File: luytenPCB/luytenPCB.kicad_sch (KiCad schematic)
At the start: 36 parts, among them IC1 DRV8212DRLR, IC2 DRV8212DRLR, J1 Battery, J10 START_M, J2 BDC1, J3 BDC2, J4 LINE_RF, J5 LINE_LF, J6 DIST_L, J7 DIST_LM, J8 DIST_R, J9 DIST_RM, SW1 SW_SPST, SW2 ProgSelect

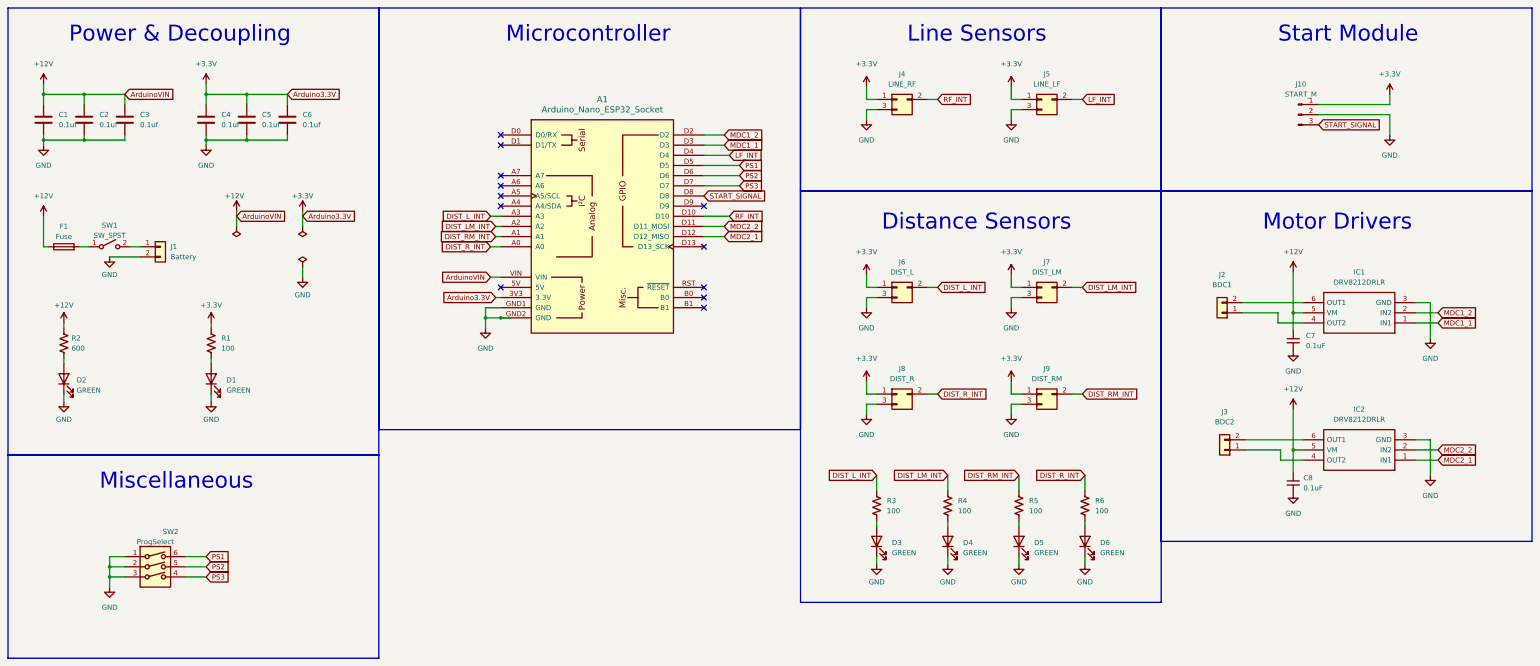
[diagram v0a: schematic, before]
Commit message: pcb production prototype done
finished schematic and layout
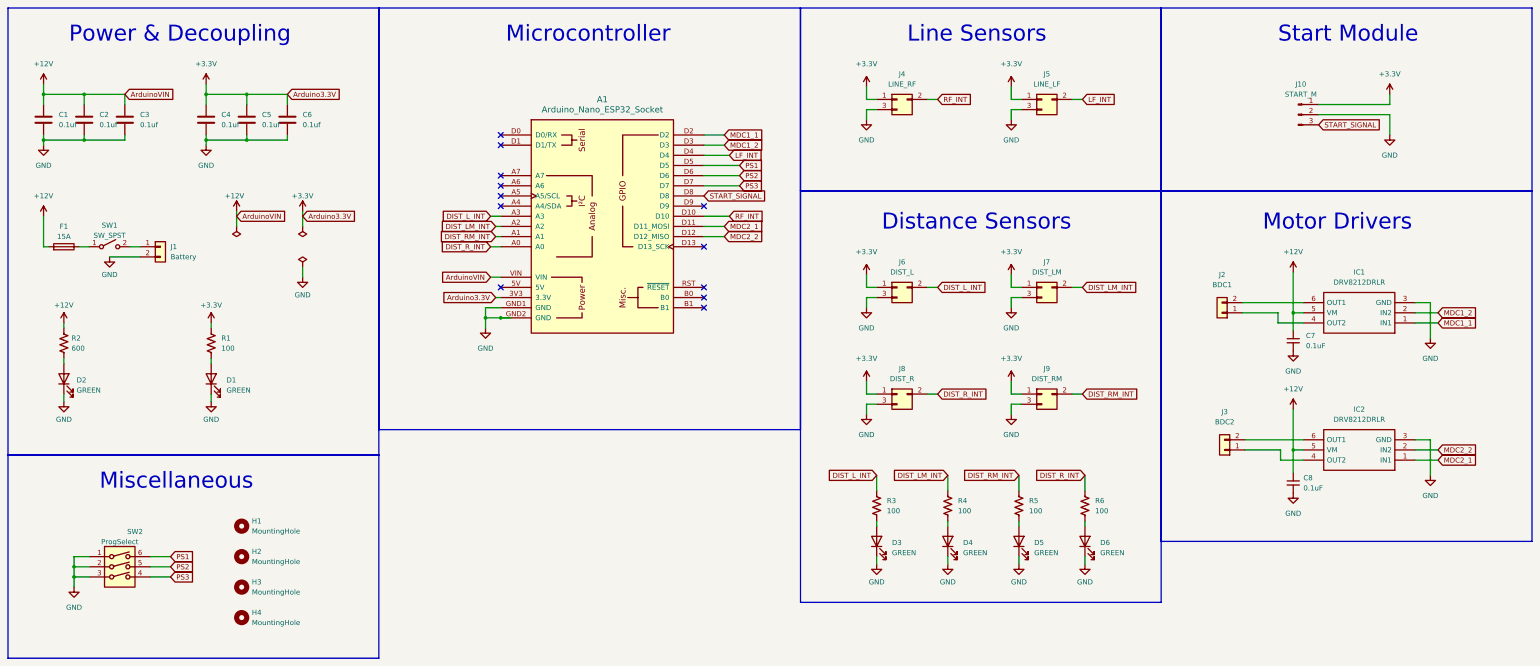
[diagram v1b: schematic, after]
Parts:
- added H1, H2, H3, H4: MountingHole, MountingHole:MountingHole_2.2mm_M2_ISO7380, symbol Mechanical:MountingHole
- F1: value Fuse -> 15A; footprint (none) -> Fuse:Fuse_1206_3216Metric_Pad1.42x1.75mm_HandSolder
- J1: footprint Connector_AMASS:AMASS_XT30PW-M_1x02_P2.50mm_Horizontal -> Connector_AMASS:AMASS_XT30U-M_1x02_P5.0mm_Vertical
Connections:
- net +12V: now also F1.2; no longer F1.1
- net MDC1_1: now also A1.D2; no longer A1.D3
- net MDC1_2: now also A1.D3; no longer A1.D2
- net MDC2_1: now also A1.D11 (D11_MOSI); no longer A1.D12 (D12_MISO)
- net MDC2_2: now also A1.D12 (D12_MISO); no longer A1.D11 (D11_MOSI)
- net at SW1.1 (A): now also F1.1; no longer F1.2
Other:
- moved on the sheet: F1, SW2

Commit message: updates
--fixes to routing, updated screw terminal
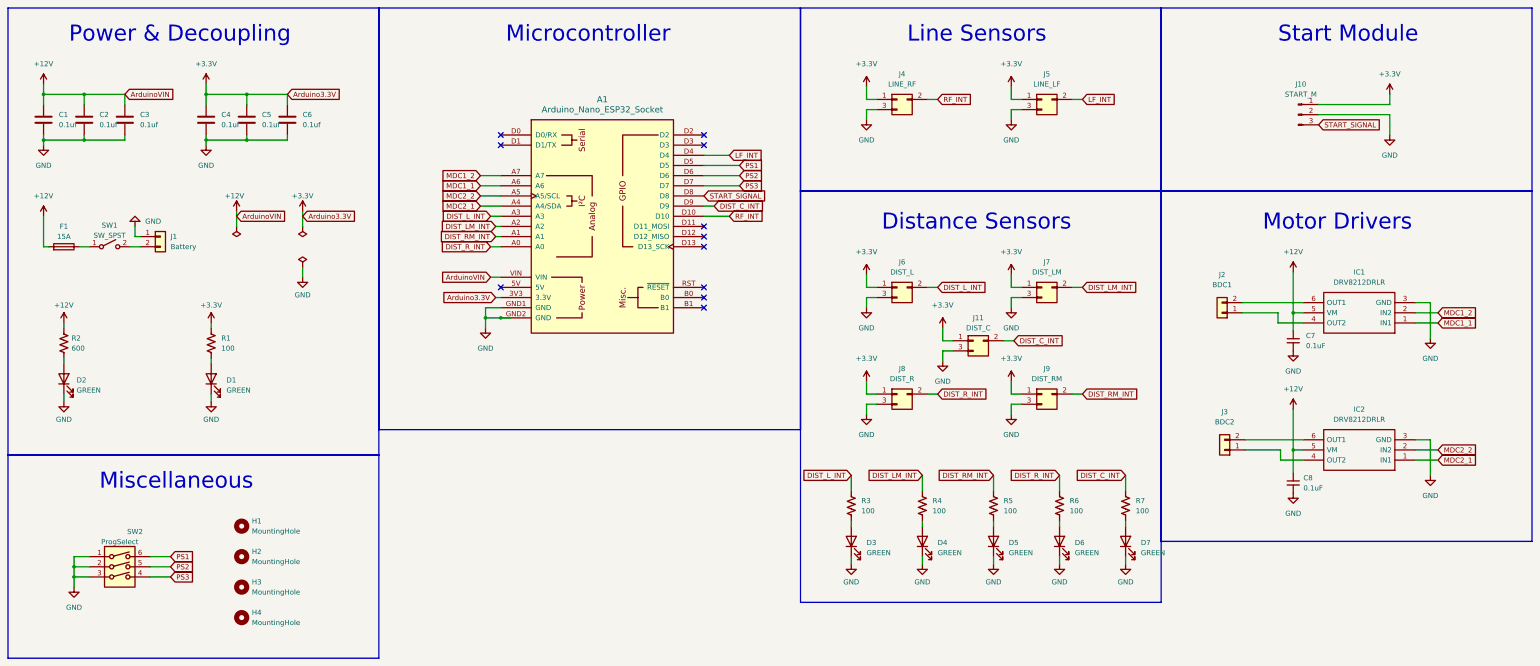
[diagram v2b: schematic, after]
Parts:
- added D7: GREEN, Capacitor_SMD:C_0603_1608Metric_Pad1.08x0.95mm_HandSolder, symbol Device:LED
- added J11: DIST_C, Connector_PinHeader_2.54mm:PinHeader_1x03_P2.54mm_Vertical, symbol Connector_Generic:Conn_02x02_Odd_Even
- added R7: 100, Diode_SMD:D_0805_2012Metric_Pad1.15x1.40mm_HandSolder, symbol Device:R_US
- J2, J3: footprint Connector_Phoenix_MSTB:PhoenixContact_MSTBA_2,5_2-G_1x02_P5.00mm_Horizontal -> Connector_PinHeader_2.54mm:PinHeader_1x02_P2.54mm_Vertical
- J4, J5, J6, J7, J8, J9: footprint Connector_Phoenix_MSTB:PhoenixContact_MSTBA_2,5_3-G_1x03_P5.00mm_Horizontal -> Connector_PinHeader_2.54mm:PinHeader_1x03_P2.54mm_Vertical
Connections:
- net +3.3V: now also J11.1 (Pin_1)
- net GND: now also J1.1 (Pin_1), D7.1 (K), J11.3 (Pin_3); no longer J1.2 (Pin_2)
- net MDC1_1: now also A1.A6; no longer A1.D2
- net MDC1_2: now also A1.A7; no longer A1.D3
- net MDC2_1: now also A1.A4 (A4/SDA); no longer A1.D11 (D11_MOSI)
- net MDC2_2: now also A1.A5 (A5/SCL); no longer A1.D12 (D12_MISO)
- net at SW1.2 (B): now also J1.2 (Pin_2); no longer J1.1 (Pin_1)
- net DIST_C_INT: now reaches A1.D9
- net DIST_C_INT: now also J11.2 (Pin_2), R7.1
- new net: D7.2 (A), R7.2
- no-connect marks 12 -> 11
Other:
- moved on the sheet: D3, D4, D5, D6, J1, R3, R4, R5, R6
